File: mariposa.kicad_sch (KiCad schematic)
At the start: 37 parts, among them J1 Conn_01x22_Shielded, J2 Conn_01x03_MountingPin, J3 Conn_ARM_SWD_TagConnect_TC203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, J6 Conn_01x10_MountingPin, J8 Conn_01x04_MountingPin, J9 Conn_02x03_Odd_Even, SW1 SW_Push, SW3 SW_Push, U4 TPS22917DBV

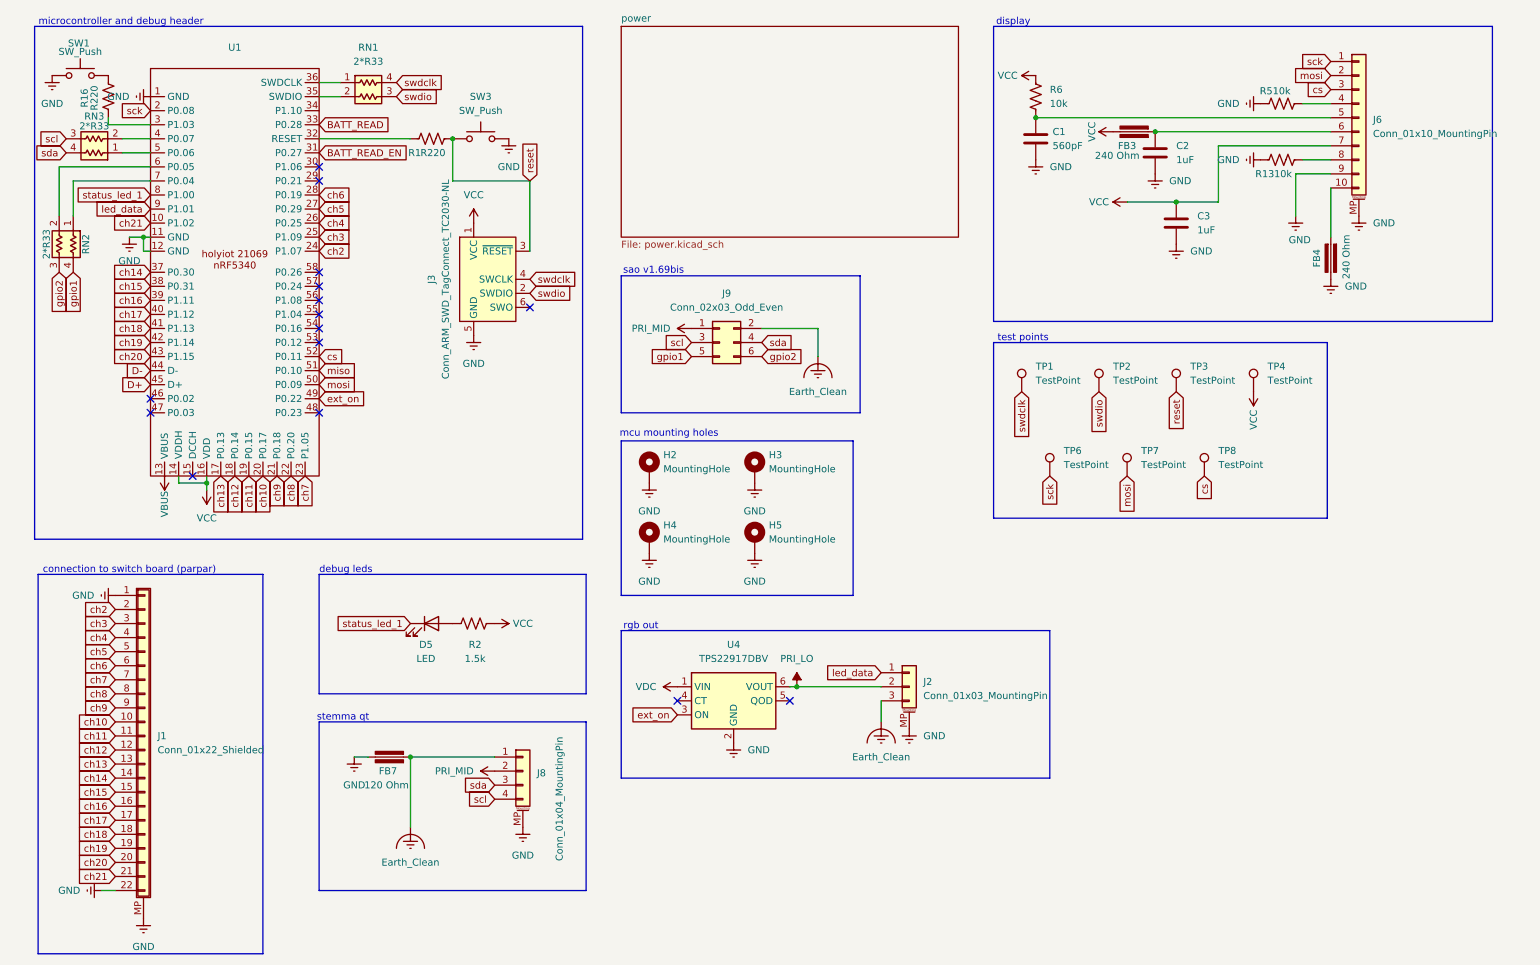
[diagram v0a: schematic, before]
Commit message: mariposa v2 pre
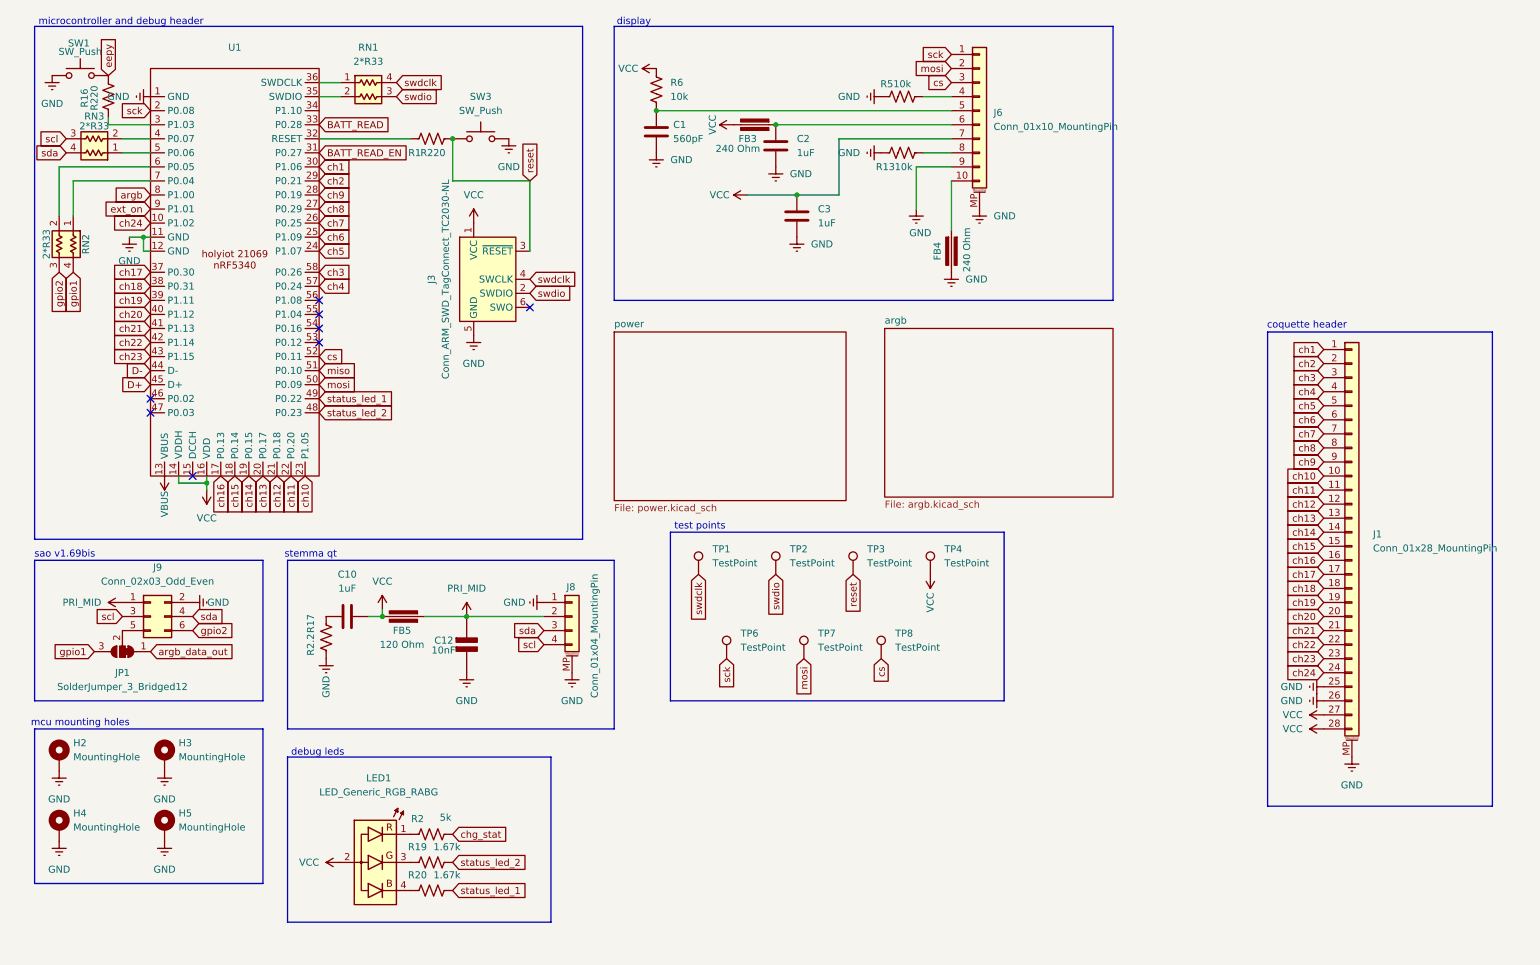
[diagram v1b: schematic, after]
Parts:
- removed D5: LED, coquette_footprints:LED 1206 reverse mount rectangle, symbol Device:LED
- removed FB7: 120 Ohm, PCM_Ferrite_SMD_AKL:Ferrite_0805_2012Metric, symbol PCM_Device_AKL:Ferrite_Bead
- removed J2: Conn_01x03_MountingPin, Connector_JST:JST_SH_SM03B-SRSS-TB_1x03-1MP_P1.00mm_Horizontal, symbol Connector_Generic_MountingPin:Conn_01x03_MountingPin
- removed U4: TPS22917DBV, Package_TO_SOT_SMD:SOT-23-6, symbol Power_Management:TPS22917DBV
- added C10: 1uF, Capacitor_SMD:C_0603_1608Metric, symbol Device:C
- added C12: 10nF, Capacitor_SMD:C_0402_1005Metric, symbol PCM_Elektuur:C
- added FB5: 120 Ohm, PCM_Ferrite_SMD_AKL:Ferrite_0805_2012Metric, symbol PCM_Device_AKL:Ferrite_Bead
- added JP1: SolderJumper_3_Bridged12, Jumper:SolderJumper-3_P1.3mm_Bridged12_RoundedPad1.0x1.5mm, symbol Jumper:SolderJumper_3_Bridged12
- added LED1: LED_Generic_RGB_RABG, coquette_footprints:E6CC1205RGBC3UDA, symbol PCM_LED_AKL:LED_Generic_RGB_RABG
- added R17: R2.2, Resistor_SMD:R_0603_1608Metric, symbol Device:R_US
- added R19, R20: 1.67k, Resistor_SMD:R_0402_1005Metric, symbol Device:R_US
- J1: value Conn_01x22_Shielded -> Conn_01x28_MountingPin; footprint Connector_FFC-FPC:Hirose_FH12-22S-0.5SH_1x22-1MP_P0.50mm_Horizontal -> coquette_footprints:AMPHENOL_SFV28R-1STE1HLF; symbol Connector_Generic_Shielded:Conn_01x22_Shielded -> Connector_Generic_MountingPin:Conn_01x28_MountingPin
- J6: footprint Connector_FFC-FPC:Hirose_FH12-10S-0.5SH_1x10-1MP_P0.50mm_Horizontal -> coquette_footprints:AMPHENOL_SFV10R-1STE1HLF
- R2: value 1.5k -> 5k; footprint Resistor_SMD:R_0603_1608Metric -> Resistor_SMD:R_0402_1005Metric
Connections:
- net Earth_Clean is gone; now on net GND: J8.1 (Pin_1), J9.2 (Pin_2)
- net led_data is gone; now on net ext_on: U1.9 (P1.01)
- net GND: now also J1.25 (Pin_25), J1.26 (Pin_26), C12.2 (-), R17.2; no longer J1.1 (Pin_1), J1.22 (Pin_22)
- net PRI_MID: now also C12.1 (+), FB5.1
- net VCC: now also J1.27 (Pin_27), J1.28 (Pin_28), C10.2, FB5.2, LED1.2 (A); no longer R2.2
- net ch10: now also U1.23 (P1.05); no longer U1.20 (P0.17)
- net ch11: now also U1.22 (P0.20); no longer U1.19 (P0.15)
- net ch12: now also U1.21 (P0.18); no longer U1.18 (P0.14)
- net ch13: now also U1.20 (P0.17); no longer U1.17 (P0.13)
- net ch14: now also U1.19 (P0.15); no longer U1.37 (P0.30)
- net ch15: now also U1.18 (P0.14); no longer U1.38 (P0.31)
- net ch16: now also U1.17 (P0.13); no longer U1.39 (P1.11)
- net ch17: now also U1.37 (P0.30); no longer U1.40 (P1.12)
- net ch18: now also U1.38 (P0.31); no longer U1.41 (P1.13)
- net ch19: now also U1.39 (P1.11); no longer U1.42 (P1.14)
- net ch2: now also U1.29 (P0.21); no longer U1.24 (P1.07)
- net ch20: now also U1.40 (P1.12); no longer U1.43 (P1.15)
- net ch21: now also U1.41 (P1.13); no longer U1.10 (P1.02)
- net ch3: now also U1.58 (P0.26); no longer U1.25 (P1.09)
- net ch4: now also U1.57 (P0.24); no longer U1.26 (P0.25)
- net ch5: now also U1.24 (P1.07); no longer U1.27 (P0.29)
- net ch6: now also U1.25 (P1.09); no longer U1.28 (P0.19)
- net ch7: now also U1.26 (P0.25); no longer U1.23 (P1.05)
- net ch8: now also U1.27 (P0.29); no longer U1.22 (P0.20)
- net ch9: now also U1.28 (P0.19); no longer U1.21 (P0.18)
- net ext_on: no longer U1.49 (P0.22)
- net gpio1: now also JP1.3 (B); no longer J9.5 (Pin_5)
- net status_led_1: now also U1.49 (P0.22), R20.2; no longer U1.8 (P1.00)
- net at R2.1: now also LED1.1 (R)
- net eepy: now reaches R16.1, SW1.2
- net ch1: now reaches U1.30 (P1.06)
- net ch1: now also J1.1 (Pin_1)
- net status_led_2: now reaches U1.48 (P0.23)
- net status_led_2: now also R19.2
- new net: J9.5 (Pin_5), JP1.2 (C)
- new net: C10.1, R17.1
- new net: LED1.3 (G), R19.1
- new net: LED1.4 (B), R20.1
- new net argb: U1.8 (P1.00)
- new net argb_data_out: JP1.1 (A)
- new net ch22: J1.22 (Pin_22), U1.42 (P1.14)
- new net ch23: J1.23 (Pin_23), U1.43 (P1.15)
- new net ch24: J1.24 (Pin_24), U1.10 (P1.02)
- new net chg_stat: R2.2
- no-connect marks 15 -> 8
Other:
- added sheet argb (argb.kicad_sch)
- note added: "coquette header"
- note removed: "connection to switch board (parpar)"
- note removed: "rgb out"
- moved on the sheet: C1, C2, C3, FB3, FB4, H2, H3, H4, H5, J6, J8, J9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
